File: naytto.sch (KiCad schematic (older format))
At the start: 53 parts, among them Q10 2N7002, Q11 2N7002, Q12 2N7002, Q13 2N7002, Q14 2N7002, Q15 BSS83P, Q16 BSS83P, Q17 BSS83P, Q2 2N7002, Q3 BSS83P, Q4 2N7002, Q5 2N7002, Q6 2N7002, Q7 2N7002, Q8 2N7002, Q9 2N7002

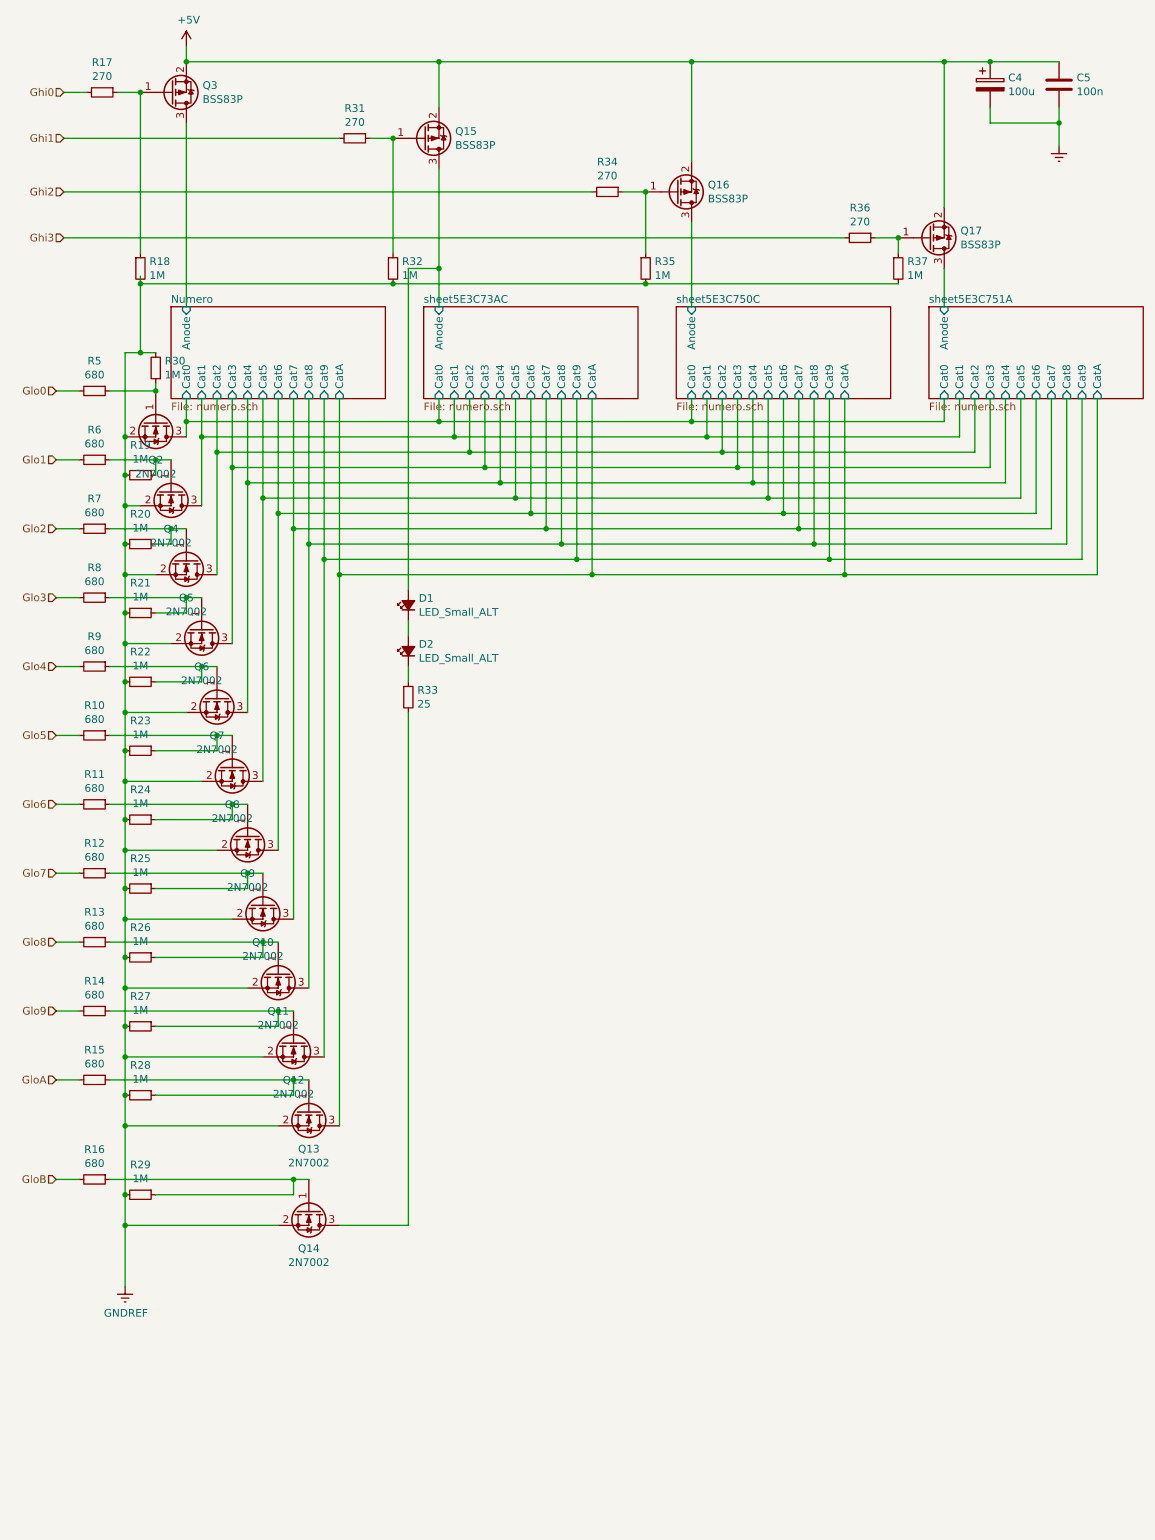
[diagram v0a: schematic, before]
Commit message: joo
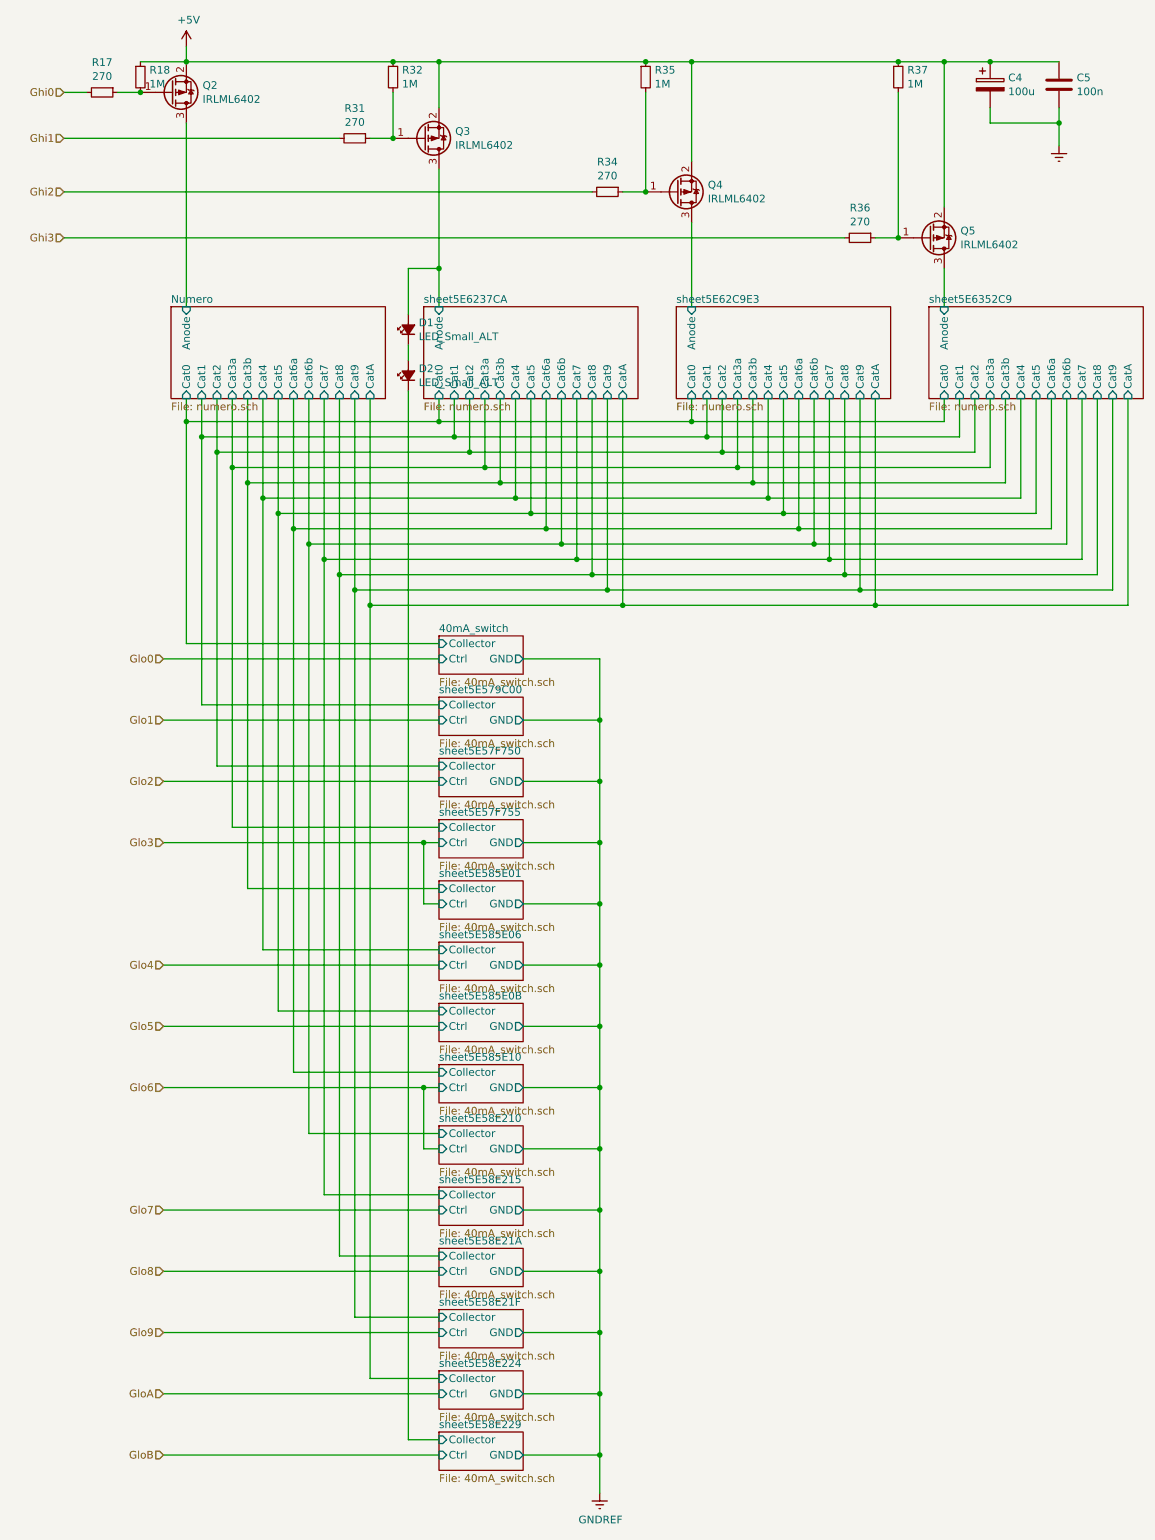
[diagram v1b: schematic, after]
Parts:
- removed Q10, Q11, Q12, Q13, Q14, Q2, Q4, Q5, Q6, Q7, Q8, Q9: 2N7002, Package_TO_SOT_SMD:SOT-416, symbol Transistor_FET:2N7002
- removed Q15, Q16, Q17, Q3: BSS83P, Package_TO_SOT_SMD:SOT-23, symbol Transistor_FET:BSS83P
- removed R10, R11, R12, R13, R14, R15, R16, R5, R6, R7, R8, R9: 680, Resistor_SMD:R_0805_2012Metric, symbol Device:R_Small
- removed R19, R20, R21, R22, R23, R24, R25, R26, R27, R28, R29, R30: 1M, Resistor_SMD:R_0805_2012Metric, symbol Device:R_Small
- removed R33: 25, Resistor_SMD:R_1206_3216Metric, symbol Device:R_Small
- added Q2, Q3, Q4, Q5: IRLML6402, Package_TO_SOT_SMD:SOT-23, symbol Transistor_FET:IRLML6402
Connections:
- net +5V: now also R18.1, R32.1, R35.1, R37.1, Q2.2 (S), Q3.2 (S), Q4.2 (S), Q5.2 (S)
- net GNDREF: no longer R18.2, R32.2, R35.2, R37.2
- net Numero/Anode: now also Q2.3 (D)
- net at R17.1: now also R18.2, Q2.1 (G); no longer R18.1
- net at R31.1: now also R32.2, Q3.1 (G); no longer R32.1
- net at R34.1: now also R35.2, Q4.1 (G); no longer R35.1
- net at R36.1: now also R37.2, Q5.1 (G); no longer R37.1
- net sheet5E58E229/Collector: now reaches D2.1 (K)
- net sheet5E3C73AC/Anode renamed sheet5E6237CA/Anode
- net sheet5E6237CA/Anode: now also Q3.3 (D)
- new net sheet5E62C9E3/Anode: Q4.3 (D)
- new net sheet5E6352C9/Anode: Q5.3 (D)
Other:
- moved on the sheet: D1, D2, R18, R32, R35, R37

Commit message: joo
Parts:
- D1, D2: footprint LED_THT:LED_D3.0mm_Clear -> LED_THT:LED_D3.0mm_Front
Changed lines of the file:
@@
 F 0 "D2" V 3696 3182 50  0000 R CNN
 F 1 "LED_Small_ALT" V 3605 3182 50  0000 R CNN
-F 2 "LED_THT:LED_D3.0mm_Clear" V 3650 3250 50  0001 C CNN
+F 2 "LED_THT:LED_D3.0mm_Front" V 3650 3250 50  0001 C CNN
 F 3 "~" V 3650 3250 50  0001 C CNN
 	1    3650 3250
@@
 F 0 "D1" V 3696 2882 50  0000 R CNN
 F 1 "LED_Small_ALT" V 3605 2882 50  0000 R CNN
-F 2 "LED_THT:LED_D3.0mm_Clear" V 3650 2950 50  0001 C CNN
+F 2 "LED_THT:LED_D3.0mm_Front" V 3650 2950 50  0001 C CNN
 F 3 "~" V 3650 2950 50  0001 C CNN
 	1    3650 2950

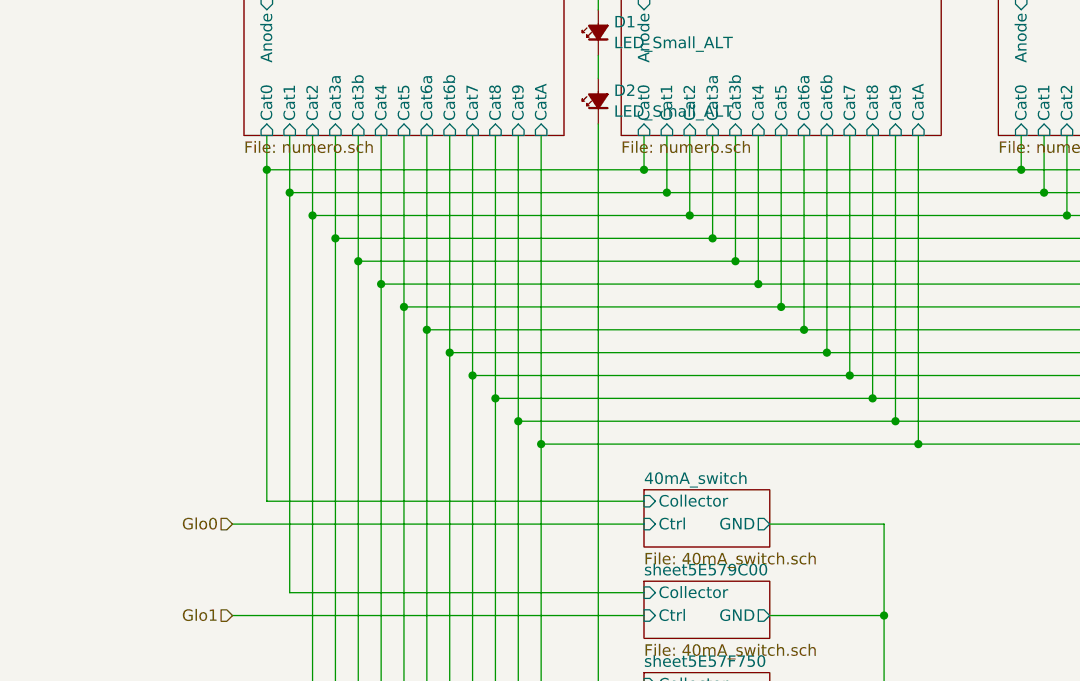
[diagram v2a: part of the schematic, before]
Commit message: joo
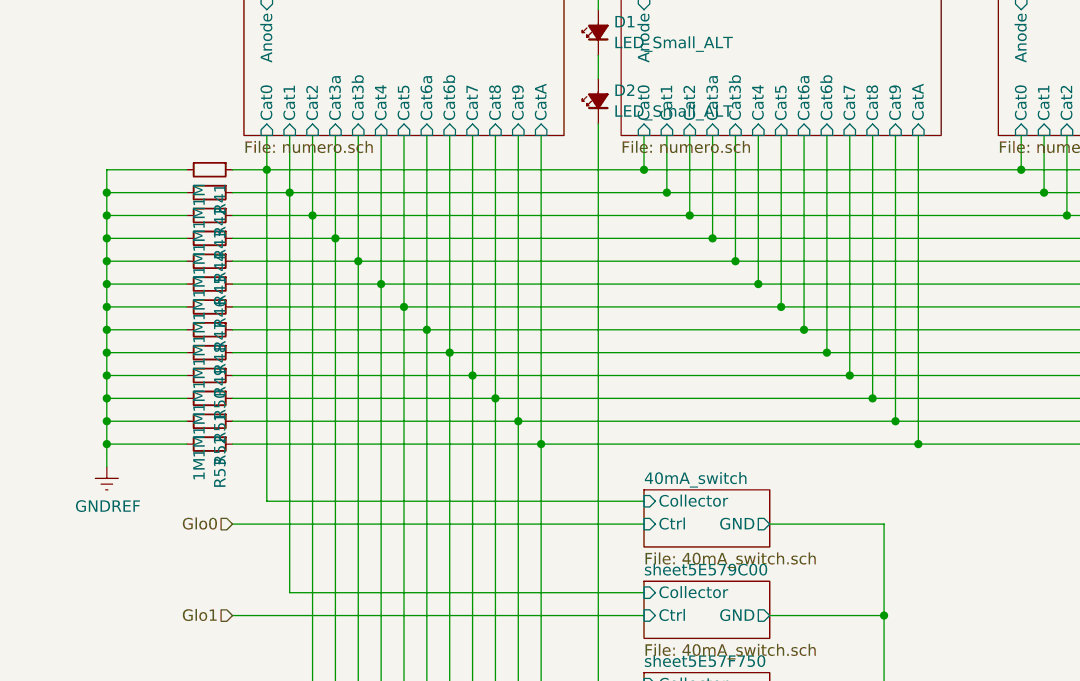
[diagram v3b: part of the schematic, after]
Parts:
- added R41, R42, R43, R44, R45, R46, R47, R48, R49, R50, R51, R52, R53: 1M, Resistor_SMD:R_0805_2012Metric, symbol Device:R_Small
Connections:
- net 40mA_switch/Collector: now also R41.1
- net GNDREF: now also R41.2, R42.2, R43.2, R44.2, R45.2, R46.2, R47.2, R48.2, R49.2, R50.2, R51.2, R52.2, R53.2
- net Numero/Cat1: now also R42.1
- net Numero/Cat2: now also R43.1
- net Numero/Cat3a: now also R44.1
- net Numero/Cat3b: now also R45.1
- net Numero/Cat4: now also R46.1
- net Numero/Cat5: now also R47.1
- net Numero/Cat6a: now also R48.1
- net Numero/Cat6b: now also R49.1
- net Numero/Cat7: now also R50.1
- net Numero/Cat8: now also R51.1
- net Numero/Cat9: now also R52.1
- net Numero/CatA: now also R53.1
